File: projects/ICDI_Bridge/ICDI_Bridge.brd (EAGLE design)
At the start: 190.5 x 60.3 mm, 8 parts

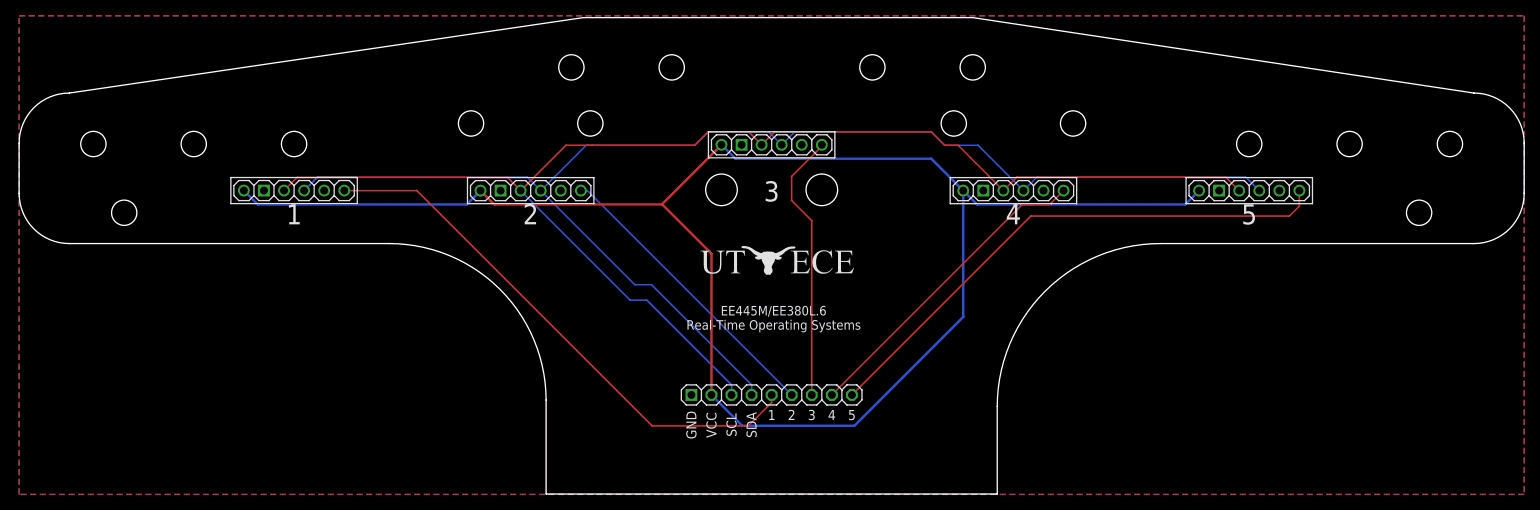
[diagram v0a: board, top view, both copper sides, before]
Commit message: April sync
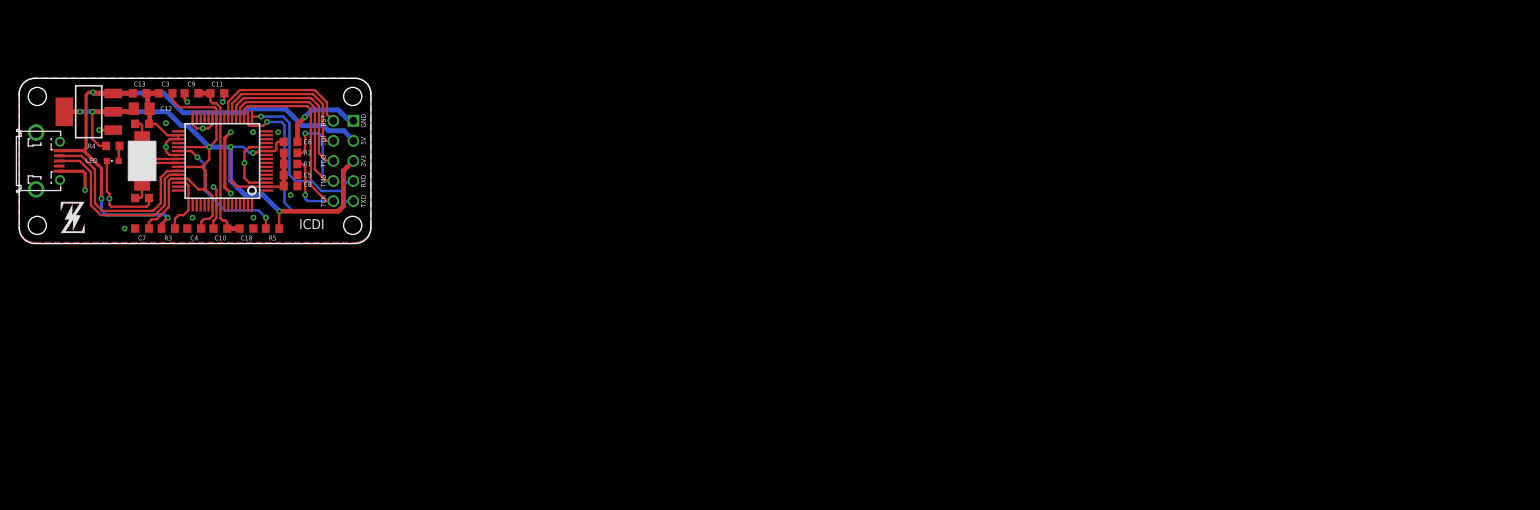
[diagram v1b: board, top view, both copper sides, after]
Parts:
- removed U$5, U$6: LIDAR_VL53L0X_ATK_VERT, Z:LIDAR_VL53L0X_ATK_VERT
- removed U$7: (no value), Z:LOGO_UT_ECE_20X4
- removed U$8: (no value), Z:LOGO_Z_3X4
- added C1, C2: 10pF, UT_ECE:C0603K
- added C10, C4, C6, C9: 0.1uF, UT_ECE:C0603K
- added C11, C7: 1uF, UT_ECE:C0603K
- added C12: (no value), UT_ECE:C0805K
- added C13: (no value), UT_ECE:C0603K
- added C18: 2.2uF, UT_ECE:C0603K
- added C3, C5, C8: 0.01uF, UT_ECE:C0603K
- added IC1: TM4C123GH6PM, UT_ECE:SQFP-S-10X10-64
- added LED: (no value), adafruit:CHIPLED_0603
- added Q1: NX5032GA, UT_ECE:NX5032GA
- added R1, R2, R4, R5: 10k, UT_ECE:R0603
- added R3: 330, UT_ECE:R0603
- U$1: value UTX_EE445M_LIDAR_FRONT_BOARD_CONNECTOR_PTH -> USB_MICRO_PTH; device Z:UTX_EE445M_LIDAR_FRONT_BOARD_CONNECTOR_PTH -> Z:USB_MICRO_PTH
- U$2: value LIDAR_VL53L0X_ATK_VERT -> JTAG_SERIAL; device Z:LIDAR_VL53L0X_ATK_VERT -> Z:JTAG_SERIAL_PTH
- U$3: value LIDAR_VL53L0X_ATK_VERT -> (none); device Z:LIDAR_VL53L0X_ATK_VERT -> Z:__LOGO_Z
- U$4: value LIDAR_VL53L0X_ATK_VERT -> _VOLTAGE_REGULATOR_AMS1117; device Z:LIDAR_VL53L0X_ATK_VERT -> Z:_PACKAGE_SOT223
- moved U$1 100.3 mm to (0.25, 10.5)
- moved U$4 86.5 mm to (8.81, 16.7), turned to 90 degrees
- moved U$3 59.7 mm to (5.25, 1.32)
- moved U$2 7.28 mm to (41.0, 10.5), turned to 90 degrees
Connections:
- removed net N$13: U$2.INT
- removed net N$3: U$4.INT
- removed net N$5: U$5.INT
- removed net SCL: U$1.SCL, U$2.SCL, U$3.SCL, U$4.SCL, U$5.SCL, U$6.SCL
- removed net SDA: U$1.SDA, U$2.SDA, U$3.SDA, U$4.SDA, U$5.SDA, U$6.SDA
- removed net VCC: U$1.VCC, U$2.VCC, U$3.VCC, U$4.VCC, U$5.VCC, U$6.VCC
- removed net XSHUT1: U$1.XSHUT1, U$2.XSH
- removed net XSHUT2: U$1.XSHUT2, U$3.XSH
- removed net XSHUT3: U$1.XSHUT3, U$4.XSH
- removed net XSHUT4: U$1.XSHUT4, U$5.XSH
- removed net XSHUT5: U$1.XSHUT5, U$6.XSH
- new net 3V3: C12.1, C3.1, C4.1, C5.1, C6.1, C7.1, C8.1, IC1.11, IC1.2, IC1.26, IC1.37, IC1.42, IC1.45, IC1.54, R1.2, R2.2, R4.2, R5.2, U$2.3V3, U$4.2, U$4.4
- new net 5V: C13.1, R3.2, U$1.1, U$2.5V, U$4.3
- new net LDO: C10.1, C11.1, C18.1, C9.1, IC1.25, IC1.56
- new net N$4: IC1.38, R5.1
- new net OSC0: C1.1, IC1.40, Q1.1
- new net OSC1: C2.1, IC1.41, Q1.2
- new net RST: IC1.23, U$2.RST
- new net TCK: IC1.19, R1.1, U$2.TCK
- new net TDI: IC1.22, U$2.TDI
- new net TDO: IC1.21, U$2.TDO
- new net TMS: IC1.20, R2.1, U$2.TMS
- new net UART0_RX: IC1.17, U$2.RXD
- new net UART0_TX: IC1.18, U$2.TXD
- new net USB_DM: IC1.43, U$1.2
- new net USB_DP: IC1.44, U$1.3
- net GND: now also C1.2, C10.2, C11.2, C12.2, C13.2, C18.2, C2.2, C3.2, C4.2, C5.2, C6.2, C7.2, C8.2, C9.2, IC1.12, IC1.27, IC1.3, IC1.32, IC1.34, IC1.35, IC1.39, IC1.55, LED.C, U$1.5, U$4.1; no longer U$1.GND, U$3.GND, U$4.GND, U$5.GND, U$6.GND
- net N$1: now also LED.A, R4.1; no longer U$3.INT
- net N$2: now also IC1.46, R3.1; no longer U$6.INT
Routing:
- net VCC: track 212.0 -> 0.00 mm
- net SDA: track 169.4 -> 0.00 mm
- net SCL: track 169.3 -> 0.00 mm
- net 3V3: track 0.00 -> 130.3 mm, vias 0 -> 6
- net GND: track 0.00 -> 75.1 mm, vias 0 -> 19
- net 5V: track 0.00 -> 71.3 mm, vias 0 -> 3
- net XSHUT1: track 68.6 -> 0.00 mm
- net XSHUT5: track 68.5 -> 0.00 mm
- net XSHUT4: track 40.0 -> 0.00 mm
- net XSHUT2: track 37.4 -> 0.00 mm
- net XSHUT3: track 34.3 -> 0.00 mm
- net TMS: track 0.00 -> 34.2 mm, vias 0 -> 1
- net TCK: track 0.00 -> 31.8 mm, vias 0 -> 1
- net UART0_TX: track 0.00 -> 25.7 mm, vias 0 -> 1
- net USB_DM: track 0.00 -> 24.4 mm
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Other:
- board size 190.5 x 60.3 mm -> 44.5 x 20.9 mm
- board text added: "ICDI"
- board text added: "Mar 2019 Zee Lv"
- board text removed: "1"
- board text removed: "2"
- board text removed: "3"
- board text removed: "4"
- board text removed: "5"
- board text removed: "EE445M/EE380L.6 Real-Time Operating Systems"
- board text removed: "University of Texas at Austin Zee Lv, Sijin Woo March 2019"
